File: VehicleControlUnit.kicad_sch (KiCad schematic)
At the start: 6 parts, among them J3 Conn_01x02, Q1 Q_PMOS_GDS

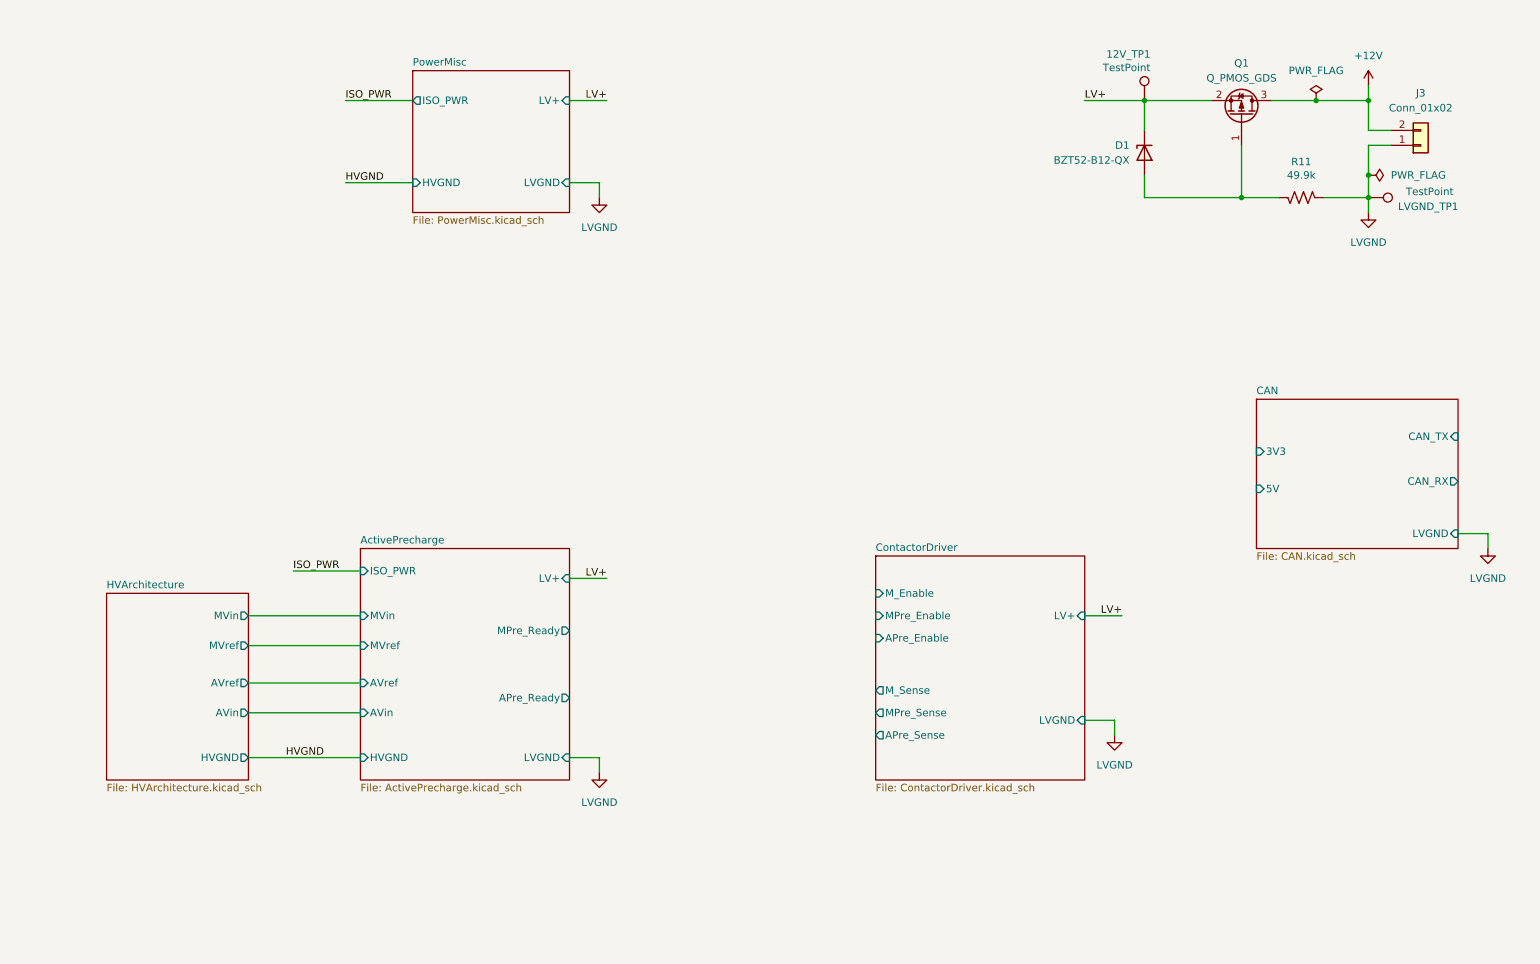
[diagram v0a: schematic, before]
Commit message: initial commit post VCU block diagram
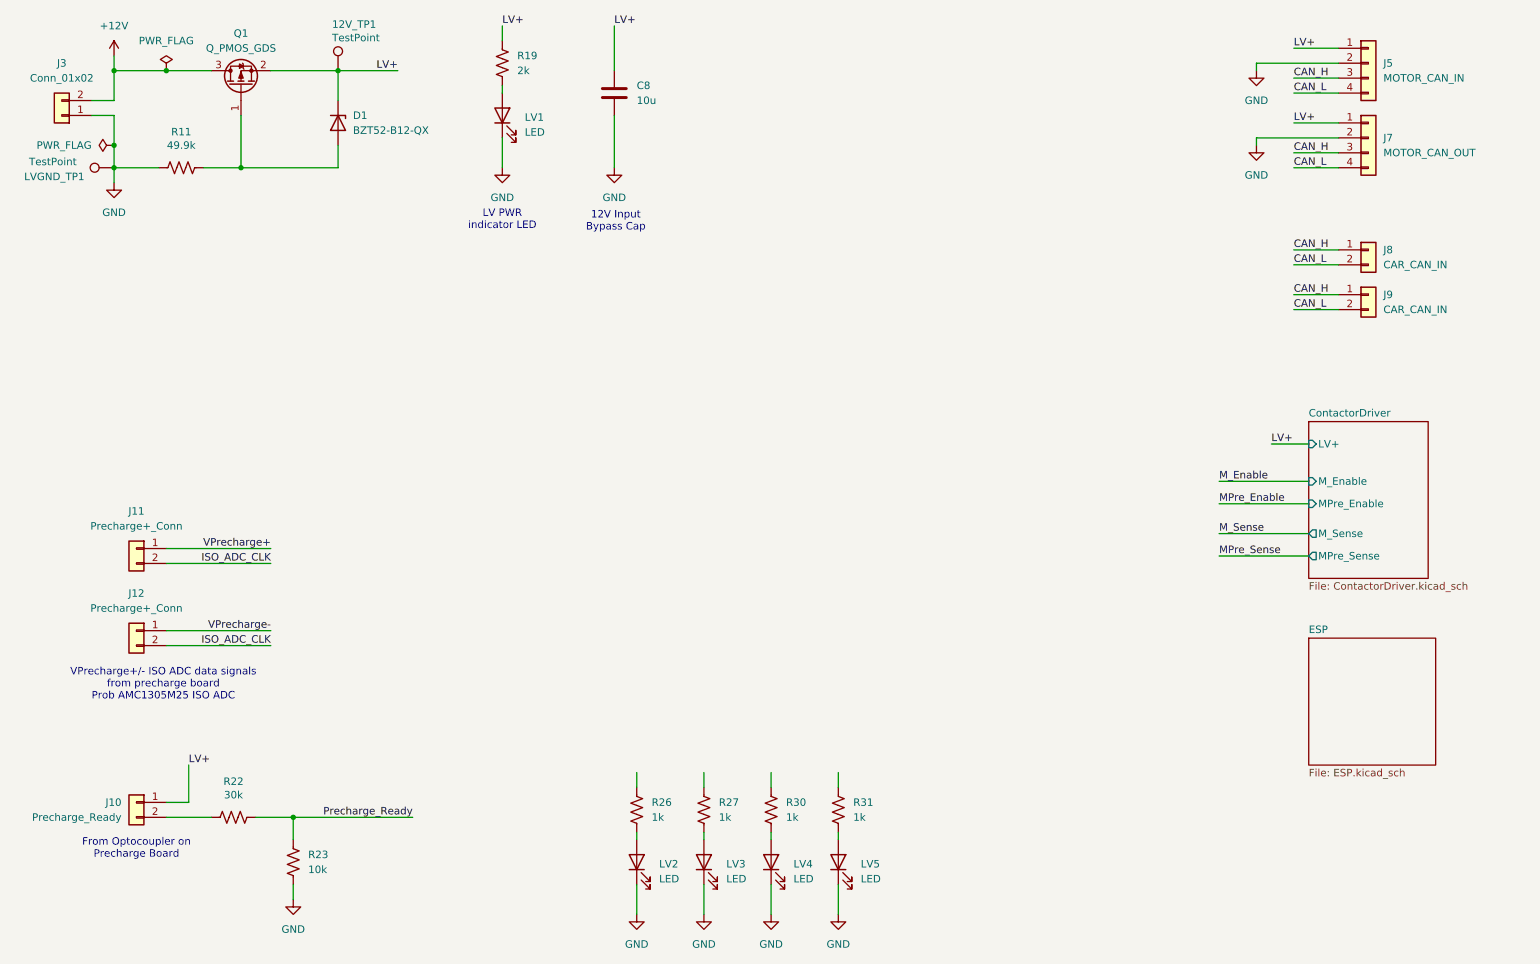
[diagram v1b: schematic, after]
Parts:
- added C8: 10u, Capacitor_SMD:C_0805_2012Metric, symbol Device:C
- added J10: Precharge_Ready, symbol Connector_Generic:Conn_01x02
- added J11, J12: Precharge+_Conn, symbol Connector_Generic:Conn_01x02
- added J5: MOTOR_CAN_IN, symbol Connector_Generic:Conn_01x04
- added J7: MOTOR_CAN_OUT, symbol Connector_Generic:Conn_01x04
- added J8, J9: CAR_CAN_IN, symbol Connector_Generic:Conn_01x02
- added LV1, LV2, LV3, LV4, LV5: LED, LED_SMD:LED_0805_2012Metric, symbol Device:LED
- added R19: 2k, Resistor_SMD:R_0805_2012Metric, symbol Device:R_US
- added R22: 30k, Resistor_SMD:R_0805_2012Metric, symbol Device:R_US
- added R23: 10k, symbol Device:R_US
- added R26, R27, R30, R31: 1k, Resistor_SMD:R_0805_2012Metric, symbol Device:R_US
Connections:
- net LV+: now also C8.1, J10.1 (Pin_1), J5.1 (Pin_1), J7.1 (Pin_1), R19.1
- net LVGND renamed GND
- net GND: now also C8.2, J5.2 (Pin_2), J7.2 (Pin_2), LV1.1 (K), LV2.1 (K), LV3.1 (K), LV4.1 (K), LV5.1 (K), R23.2
- new net: LV4.2 (A), R30.2
- new net: LV2.2 (A), R26.2
- new net: J10.2 (Pin_2), R22.1
- new net: LV5.2 (A), R31.2
- new net: LV3.2 (A), R27.2
- new net: LV1.2 (A), R19.2
- new net CAN_H: J5.3 (Pin_3), J7.3 (Pin_3), J8.1 (Pin_1), J9.1 (Pin_1)
- new net CAN_L: J5.4 (Pin_4), J7.4 (Pin_4), J8.2 (Pin_2), J9.2 (Pin_2)
- new net ISO_ADC_CLK: J11.2 (Pin_2), J12.2 (Pin_2)
- new net Precharge_Ready: R22.2, R23.1
- new net VPrecharge+: J11.1 (Pin_1)
- new net VPrecharge-: J12.1 (Pin_1)
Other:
- removed sheet ActivePrecharge
- removed sheet CAN
- removed sheet HVArchitecture
- removed sheet PowerMisc
- added sheet ESP (ESP.kicad_sch)
- sheet ContactorDriver ports: added none; removed APre_Enable, APre_Sense, LVGND
- note added: "12V Input Bypass Cap"
- note added: "From Optocoupler on Precharge Board"
- note added: "LV PWR indicator LED"
- note added: "VPrecharge+/- ISO ADC data signals from precharge board Prob AMC1305M25 ISO ADC"
- moved on the sheet: 12V_TP1, D1, J3, LVGND_TP1, Q1, R11
